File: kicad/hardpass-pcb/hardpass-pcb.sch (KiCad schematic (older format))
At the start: 55 parts, among them P1 Pi_Zero, P2 OLED_I2C, SW1 1, SW10 C/UP, SW11 0/OK, SW12 OK/DN, SW13 SHUTDN, SW14 SW_PUSH_SMALL, SW2 2, SW3 3, SW4 4, SW5 5, SW6 6, SW7 7, SW8 8, SW9 9, U1 ISO7816, U2 ESP-12E, U3 TDA8029, Y1 14.745MHz

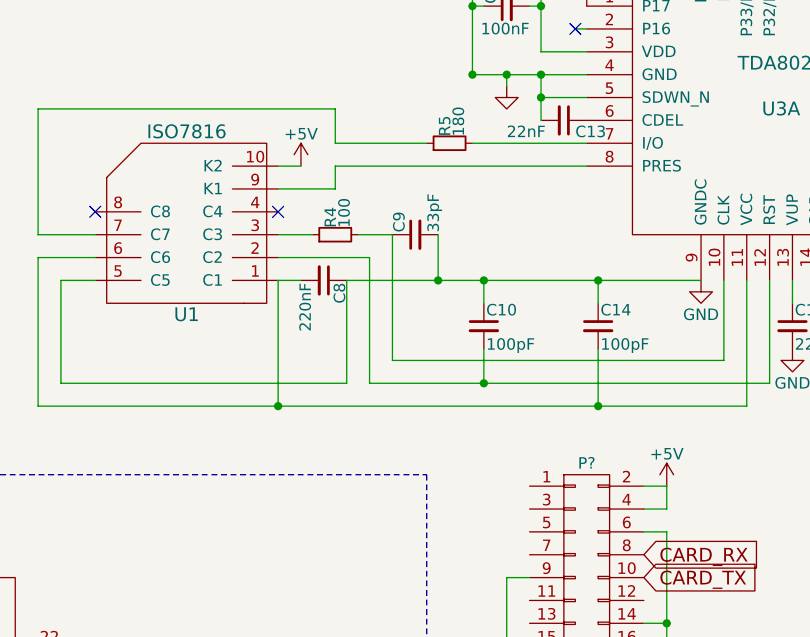
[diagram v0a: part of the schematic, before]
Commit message: routed 2nd board
not finished, but a start
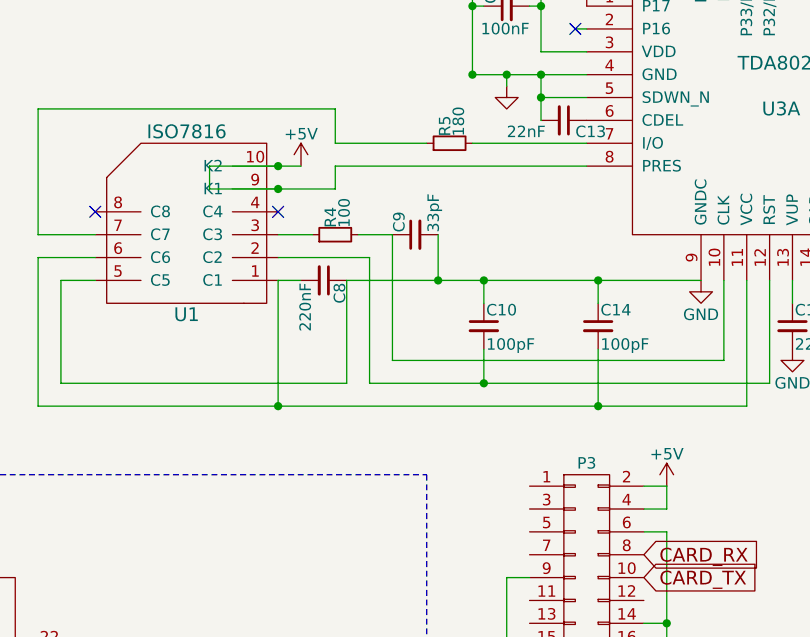
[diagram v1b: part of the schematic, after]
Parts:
- P3: renamed from P?; footprint Pin_Headers:Pin_Header_Straight_2x20_Pitch2.54mm -> hardpass:Pin_Header_Straight_2x20_Pitch2.54mm_centered
- Y1: footprint (none) -> Crystals:Crystal_HC49-U_Vertical
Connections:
- net +5V: now also U1.9 (K1), U3.8 (PRES)
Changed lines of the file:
@@
 ROW_4
 $Comp
-L GND #PWR1
+L GND #PWR01
 U 1 1 57211ADA
 P 1000 3100
-F 0 "#PWR1" H 1000 2850 50  0001 C CNN
+F 0 "#PWR01" H 1000 2850 50  0001 C CNN
 F 1 "GND" H 1000 2950 50  0000 C CNN
 F 2 "" H 1000 3100 50  0000 C CNN
@@
 $EndComp
 $Comp
-L +3.3V #PWR2
+L +3.3V #PWR02
 U 1 1 57211B7B
 P 1050 950
-F 0 "#PWR2" H 1050 800 50  0001 C CNN
+F 0 "#PWR02" H 1050 800 50  0001 C CNN
 F 1 "+3.3V" H 1050 1090 50  0000 C CNN
 F 2 "" H 1050 950 50  0000 C CNN
@@
 SD_D1
 $Comp
-L GND #PWR3
+L GND #PWR03
 U 1 1 5723909B
 P 3000 3100
-F 0 "#PWR3" H 3000 2850 50  0001 C CNN
+F 0 "#PWR03" H 3000 2850 50  0001 C CNN
 F 1 "GND" H 3000 2950 50  0000 C CNN
 F 2 "" H 3000 3100 50  0000 C CNN
@@
 $EndComp
 $Comp
-L GND #PWR15
+L GND #PWR04
 U 1 1 576AFDF4
 P 5150 900
-F 0 "#PWR15" H 5150 650 50  0001 C CNN
+F 0 "#PWR04" H 5150 650 50  0001 C CNN
 F 1 "GND" H 5150 750 50  0001 C CNN
 F 2 "" H 5150 900 50  0000 C CNN
@@
 OLED_SCL
 $Comp
-L +3.3V #PWR12
+L +3.3V #PWR05
 U 1 1 576B9B60
 P 4850 2650
-F 0 "#PWR12" H 4850 2500 50  0001 C CNN
+F 0 "#PWR05" H 4850 2500 50  0001 C CNN
 F 1 "+3.3V" H 4850 2790 50  0001 C CNN
 F 2 "" H 4850 2650 50  0000 C CNN
@@
 $EndComp
 $Comp
-L GND #PWR13
+L GND #PWR06
 U 1 1 576B9D6C
 P 4950 3950
-F 0 "#PWR13" H 4950 3700 50  0001 C CNN
+F 0 "#PWR06" H 4950 3700 50  0001 C CNN
 F 1 "GND" H 4950 3800 50  0001 C CNN
 F 2 "" H 4950 3950 50  0000 C CNN
@@
 SHUTDOWN
 $Comp
-L GND #PWR4
+L GND #PWR07
 U 1 1 57716417
 P 3800 7050
-F 0 "#PWR4" H 3800 6800 50  0001 C CNN
+F 0 "#PWR07" H 3800 6800 50  0001 C CNN
 F 1 "GND" H 3800 6900 50  0000 C CNN
 F 2 "" H 3800 7050 50  0000 C CNN
@@
 Wifi Pants: \n    pin 27-->
 $Comp
-L GND #PWR6
+L GND #PWR08
 U 1 1 58333C64
 P 4500 1850
-F 0 "#PWR6" H 4500 1600 50  0001 C CNN
+F 0 "#PWR08" H 4500 1600 50  0001 C CNN
 F 1 "GND" H 4500 1700 50  0001 C CNN
 F 2 "" H 4500 1850 50  0000 C CNN
@@
 $EndComp
 $Comp
-L +3.3V #PWR11
+L +3.3V #PWR09
 U 1 1 58333EC0
 P 4700 1850
-F 0 "#PWR11" H 4700 1700 50  0001 C CNN
+F 0 "#PWR09" H 4700 1700 50  0001 C CNN
 F 1 "+3.3V" H 4700 1990 50  0001 C CNN
 F 2 "" H 4700 1850 50  0000 C CNN
@@
 $EndComp
 $Comp
-L +3.3V #PWR7
+L +3.3V #PWR010
 U 1 1 58337E9C
 P 4550 2150
-F 0 "#PWR7" H 4550 2000 50  0001 C CNN
+F 0 "#PWR010" H 4550 2000 50  0001 C CNN
 F 1 "+3.3V" H 4550 2290 50  0001 C CNN
 F 2 "" H 4550 2150 50  0000 C CNN
@@
 $EndComp
 $Comp
-L GND #PWR8
+L GND #PWR011
 U 1 1 58337F0D
 P 4550 2550
-F 0 "#PWR8" H 4550 2300 50  0001 C CNN
+F 0 "#PWR011" H 4550 2300 50  0001 C CNN
 F 1 "GND" H 4550 2400 50  0001 C CNN
 F 2 "" H 4550 2550 50  0000 C CNN
@@
 NoConn ~ 6600 5500
 $Comp
-L GND #PWR19
+L GND #PWR012
 U 1 1 57B89D14
 P 6600 5700
-F 0 "#PWR19" H 6600 5450 50  0001 C CNN
+F 0 "#PWR012" H 6600 5450 50  0001 C CNN
 F 1 "GND" H 6600 5550 50  0000 C CNN
 F 2 "" H 6600 5700 50  0000 C CNN
@@
 NoConn ~ 4800 5100
 $Comp
-L +3V3 #PWR9
+L +3V3 #PWR013
 U 1 1 57B89D90
 P 4600 5700
-F 0 "#PWR9" H 4600 5550 50  0001 C CNN
+F 0 "#PWR013" H 4600 5550 50  0001 C CNN
 F 1 "+3V3" H 4600 5840 50  0000 C CNN
 F 2 "" H 4600 5700 50  0000 C CNN
@@
 $EndComp
 $Comp
-L GND #PWR5
+L GND #PWR014
 U 1 1 5870295E
 P 4500 1550
-F 0 "#PWR5" H 4500 1300 50  0001 C CNN
+F 0 "#PWR014" H 4500 1300 50  0001 C CNN
 F 1 "GND" H 4500 1400 50  0001 C CNN
 F 2 "" H 4500 1550 50  0000 C CNN
@@
 $EndComp
 $Comp
-L +3.3V #PWR10
+L +3.3V #PWR015
 U 1 1 58702964
 P 4700 1550
-F 0 "#PWR10" H 4700 1400 50  0001 C CNN
+F 0 "#PWR015" H 4700 1400 50  0001 C CNN
 F 1 "+3.3V" H 4700 1690 50  0001 C CNN
 F 2 "" H 4700 1550 50  0000 C CNN
@@
 NoConn ~ 5250 1650
 $Comp
-L GND #PWR14
+L GND #PWR016
 U 1 1 58702A61
 P 5000 2000
-F 0 "#PWR14" H 5000 1750 50  0001 C CNN
+F 0 "#PWR016" H 5000 1750 50  0001 C CNN
 F 1 "GND" H 5000 1850 50  0001 C CNN
 F 2 "" H 5000 2000 50  0000 C CNN
@@
 $EndComp
 $Comp
-L +3.3V #PWR17
+L +3.3V #PWR017
 U 1 1 58702DF8
 P 5150 2100
-F 0 "#PWR17" H 5150 1950 50  0001 C CNN
+F 0 "#PWR017" H 5150 1950 50  0001 C CNN
 F 1 "+3.3V" H 5150 2240 50  0001 C CNN
 F 2 "" H 5150 2100 50  0000 C CNN
@@
 $EndComp
 $Comp
-L GND #PWR16
+L GND #PWR018
 U 1 1 58702F8A
 P 5150 1700
-F 0 "#PWR16" H 5150 1450 50  0001 C CNN
+F 0 "#PWR018" H 5150 1450 50  0001 C CNN
 F 1 "GND" H 5150 1550 50  0001 C CNN
 F 2 "" H 5150 1700 50  0000 C CNN
@@
 $EndComp
 $Comp
-L GND #PWR18
+L GND #PWR019
 U 1 1 58705FA1
 P 5150 2450
-F 0 "#PWR18" H 5150 2200 50  0001 C CNN
+F 0 "#PWR019" H 5150 2200 50  0001 C CNN
 F 1 "GND" H 5150 2300 50  0001 C CNN
 F 2 "" H 5150 2450 50  0000 C CNN
@@
 NoConn ~ 9600 1700
 $Comp
-L GND #PWR29
+L GND #PWR020
 U 1 1 5880D50E
 P 10150 1700
-F 0 "#PWR29" H 10150 1450 50  0001 C CNN
+F 0 "#PWR020" H 10150 1450 50  0001 C CNN
 F 1 "GND" H 10150 1550 50  0000 C CNN
 F 2 "" H 10150 1700 50  0000 C CNN
@@
 $EndComp
 $Comp
-L GND #PWR33
+L GND #PWR021
 U 1 1 5881377E
 P 10900 2600
-F 0 "#PWR33" H 10900 2350 50  0001 C CNN
+F 0 "#PWR021" H 10900 2350 50  0001 C CNN
 F 1 "GND" H 10900 2450 50  0000 C CNN
 F 2 "" H 10900 2600 50  0000 C CNN
@@
 $EndComp
 $Comp
-L GND #PWR26
+L GND #PWR022
 U 1 1 5881836B
 P 9700 3700
-F 0 "#PWR26" H 9700 3450 50  0001 C CNN
+F 0 "#PWR022" H 9700 3450 50  0001 C CNN
 F 1 "GND" H 9700 3550 50  0000 C CNN
 F 2 "" H 9700 3700 50  0000 C CNN
@@
 $EndComp
 $Comp
-L GND #PWR21
+L GND #PWR023
 U 1 1 5881F197
 P 8450 2550
-F 0 "#PWR21" H 8450 2300 50  0001 C CNN
+F 0 "#PWR023" H 8450 2300 50  0001 C CNN
 F 1 "GND" H 8450 2400 50  0001 C CNN
 F 2 "" H 8450 2550 50  0000 C CNN
@@
 $EndComp
 $Comp
-L GND #PWR28
+L GND #PWR024
 U 1 1 58833208
 P 10000 4200
-F 0 "#PWR28" H 10000 3950 50  0001 C CNN
+F 0 "#PWR024" H 10000 3950 50  0001 C CNN
 F 1 "GND" H 10000 4050 50  0000 C CNN
 F 2 "" H 10000 4200 50  0000 C CNN
@@
 TODO: less Caps?
 $Comp
-L GND #PWR24
+L GND #PWR025
 U 1 1 58839D11
 P 9300 3400
-F 0 "#PWR24" H 9300 3150 50  0001 C CNN
+F 0 "#PWR025" H 9300 3150 50  0001 C CNN
 F 1 "GND" H 9300 3250 50  0000 C CNN
 F 2 "" H 9300 3400 50  0000 C CNN
@@
 F 0 "Y1" H 9850 1450 50  0000 C CNN
 F 1 "14.745MHz" H 9850 1150 50  0000 C CNN
-F 2 "" H 9850 1300 50  0000 C CNN
+F 2 "Crystals:Crystal_HC49-U_Vertical" H 9850 1300 50  0001 C CNN
 F 3 "" H 9850 1300 50  0000 C CNN
 	1    9850 1300
@@
 $EndComp
 $Comp
-L GND #PWR27
+L GND #PWR026
 U 1 1 5883AC0F
 P 9850 900
-F 0 "#PWR27" H 9850 650 50  0001 C CNN
+F 0 "#PWR026" H 9850 650 50  0001 C CNN
 F 1 "GND" H 9850 750 50  0000 C CNN
 F 2 "" H 9850 900 50  0000 C CNN
@@
 $EndComp
 $Comp
-L GND #PWR32
+L GND #PWR027
 U 1 1 5883C802
 P 10650 2800
-F 0 "#PWR32" H 10650 2550 50  0001 C CNN
+F 0 "#PWR027" H 10650 2550 50  0001 C CNN
 F 1 "GND" H 10650 2650 50  0000 C CNN
 F 2 "" H 10650 2800 50  0000 C CNN
@@
 possible driver: https://github.com/larytet/TDA8029
 $Comp
-L +5V #PWR22
+L +5V #PWR028
 U 1 1 588108E7
 P 8600 1950
-F 0 "#PWR22" H 8600 1800 50  0001 C CNN
+F 0 "#PWR028" H 8600 1800 50  0001 C CNN
 F 1 "+5V" H 8600 2090 50  0000 C CNN
 F 2 "" H 8600 1950 50  0000 C CNN
@@
 $EndComp
 $Comp
-L +5V #PWR23
+L +5V #PWR029
 U 1 1 58810991
 P 8800 2200
-F 0 "#PWR23" H 8800 2050 50  0001 C CNN
+F 0 "#PWR029" H 8800 2050 50  0001 C CNN
 F 1 "+5V" H 8800 2340 50  0000 C CNN
 F 2 "" H 8800 2200 50  0000 C CNN
@@
 $EndComp
 $Comp
-L +5V #PWR31
+L +5V #PWR030
 U 1 1 58810A71
 P 10650 2500
-F 0 "#PWR31" H 10650 2350 50  0001 C CNN
+F 0 "#PWR030" H 10650 2350 50  0001 C CNN
 F 1 "+5V" H 10650 2640 50  0000 C CNN
 F 2 "" H 10650 2500 50  0000 C CNN
@@
 $EndComp
 $Comp
-L +5V #PWR30
+L +5V #PWR031
 U 1 1 58810B51
 P 10200 3400
-F 0 "#PWR30" H 10200 3250 50  0001 C CNN
+F 0 "#PWR031" H 10200 3250 50  0001 C CNN
 F 1 "+5V" H 10200 3540 50  0000 C CNN
 F 2 "" H 10200 3400 50  0000 C CNN
@@
 $EndComp
 $Comp
-L +5V #PWR25
+L +5V #PWR032
 U 1 1 588110F4
 P 9500 1500
-F 0 "#PWR25" H 9500 1350 50  0001 C CNN
+F 0 "#PWR032" H 9500 1350 50  0001 C CNN
 F 1 "+5V" H 9500 1640 50  0000 C CNN
 F 2 "" H 9500 1500 50  0000 C CNN
@@
 $EndComp
 $Comp
-L +5V #PWR20
+L +5V #PWR033
 U 1 1 588119E7
 P 7550 2900
-F 0 "#PWR20" H 7550 2750 50  0001 C CNN
+F 0 "#PWR033" H 7550 2750 50  0001 C CNN
 F 1 "+5V" H 7550 3040 50  0000 C CNN
 F 2 "" H 7550 2900 50  0000 C CNN
@@
 http://www.linkconn.com/en/product/\ne08f128a-897a-4361-86f3-81b7a41ba7d4\n'sim card samsung i9000 n7000'
 $Comp
-L CONN_02X20 P?
+L CONN_02X20 P3
 U 1 1 5881588C
 P 8800 5250
-F 0 "P?" H 8800 6300 50  0000 C CNN
+F 0 "P3" H 8800 6300 50  0000 C CNN
 F 1 "Pi_Zero" V 8800 5250 50  0000 C CNN
-F 2 "Pin_Headers:Pin_Header_Straight_2x20_Pitch2.54mm" H 8800 3900 50  0001 C CNN
+F 2 "hardpass:Pin_Header_Straight_2x20_Pitch2.54mm_centered" H 8800 3900 50  0001 C CNN
 F 3 "" H 8800 4300 50  0000 C CNN
 	1    8800 5250
@@
 $EndComp
 $Comp
-L +5V #PWR?
+L +5V #PWR034
 U 1 1 58817164
 P 9150 4300
-F 0 "#PWR?" H 9150 4150 50  0001 C CNN
+F 0 "#PWR034" H 9150 4150 50  0001 C CNN
 F 1 "+5V" H 9150 4440 50  0000 C CNN
 F 2 "" H 9150 4300 50  0000 C CNN
@@
 $EndComp
 $Comp
-L GND #PWR?
+L GND #PWR035
 U 1 1 5881733E
 P 8450 6200
-F 0 "#PWR?" H 8450 5950 50  0001 C CNN
+F 0 "#PWR035" H 8450 5950 50  0001 C CNN
 F 1 "GND" H 8450 6050 50  0000 C CNN
 F 2 "" H 8450 6200 50  0000 C CNN
@@
 $EndComp
 $Comp
-L GND #PWR?
+L GND #PWR036
 U 1 1 588173EB
 P 9150 6200
-F 0 "#PWR?" H 9150 5950 50  0001 C CNN
+F 0 "#PWR036" H 9150 5950 50  0001 C CNN
 F 1 "GND" H 9150 6050 50  0000 C CNN
 F 2 "" H 9150 6200 50  0000 C CNN
@@
 	7750 3400 9300 3400
 Wire Wire Line
-	7700 3000 7450 3000
-Wire Wire Line
-	7700 2900 7700 3000
-Wire Wire Line
-	8800 2900 7700 2900
+	7150 3000 7700 3000
+Wire Wire Line
+	7700 3000 7700 2900
+Wire Wire Line
+	7700 2900 8800 2900
 Wire Wire Line
 	7700 2800 7700 2650
@@
 Connection ~ 8600 2600
 Wire Wire Line
-	7450 2900 7550 2900
+	7150 2900 7550 2900
 Wire Wire Line
 	7450 3200 7600 3200
@@
 Wire Notes Line
 	6150 650  6150 4250
+Wire Wire Line
+	7150 3000 7150 2900
+Connection ~ 7450 2900
+Connection ~ 7450 3000
 $EndSCHEMATC
